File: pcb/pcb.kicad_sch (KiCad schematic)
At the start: 24 parts, among them U1 1117-3.3, U2 NORTH, U3 SOUTH, U4 EAST, U5 WEST

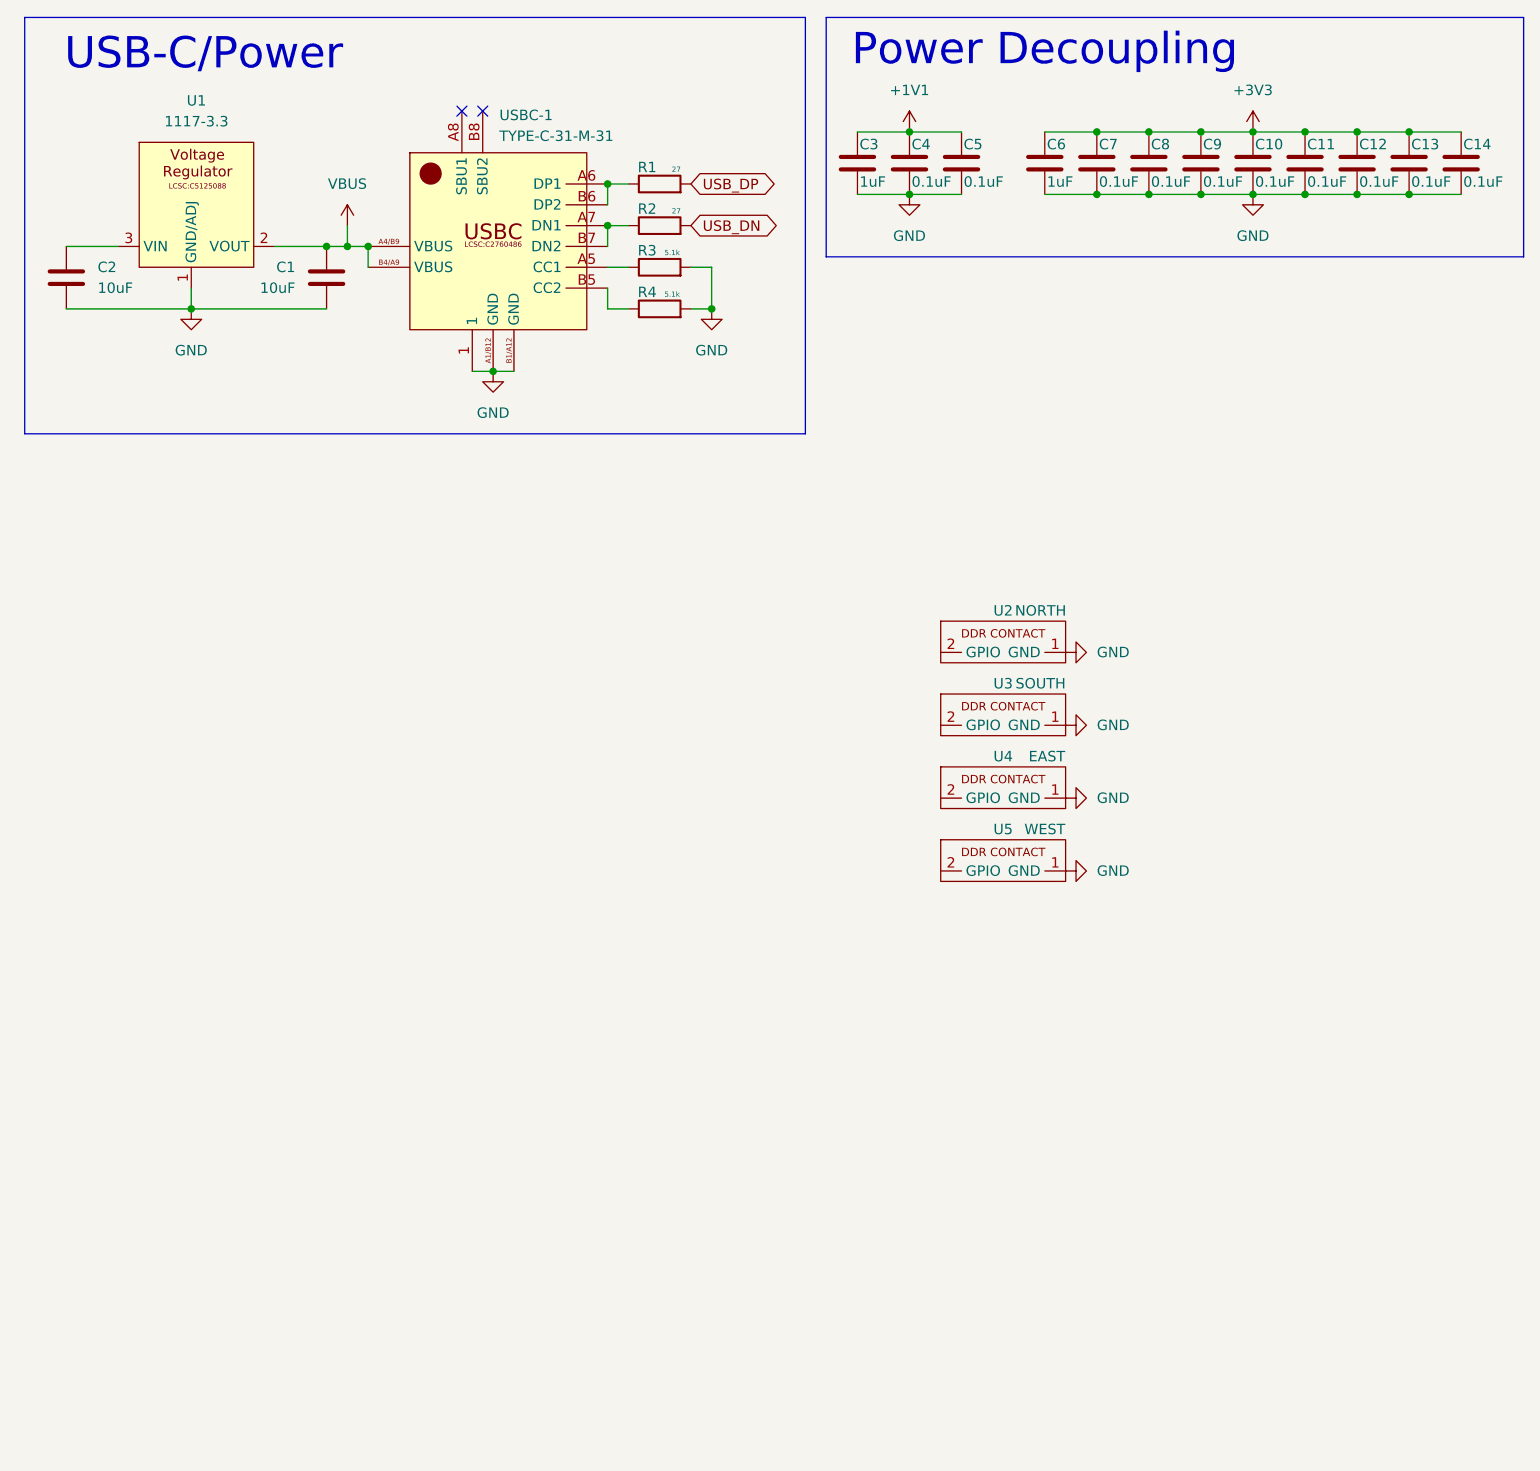
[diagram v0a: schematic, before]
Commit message: work on schematic more
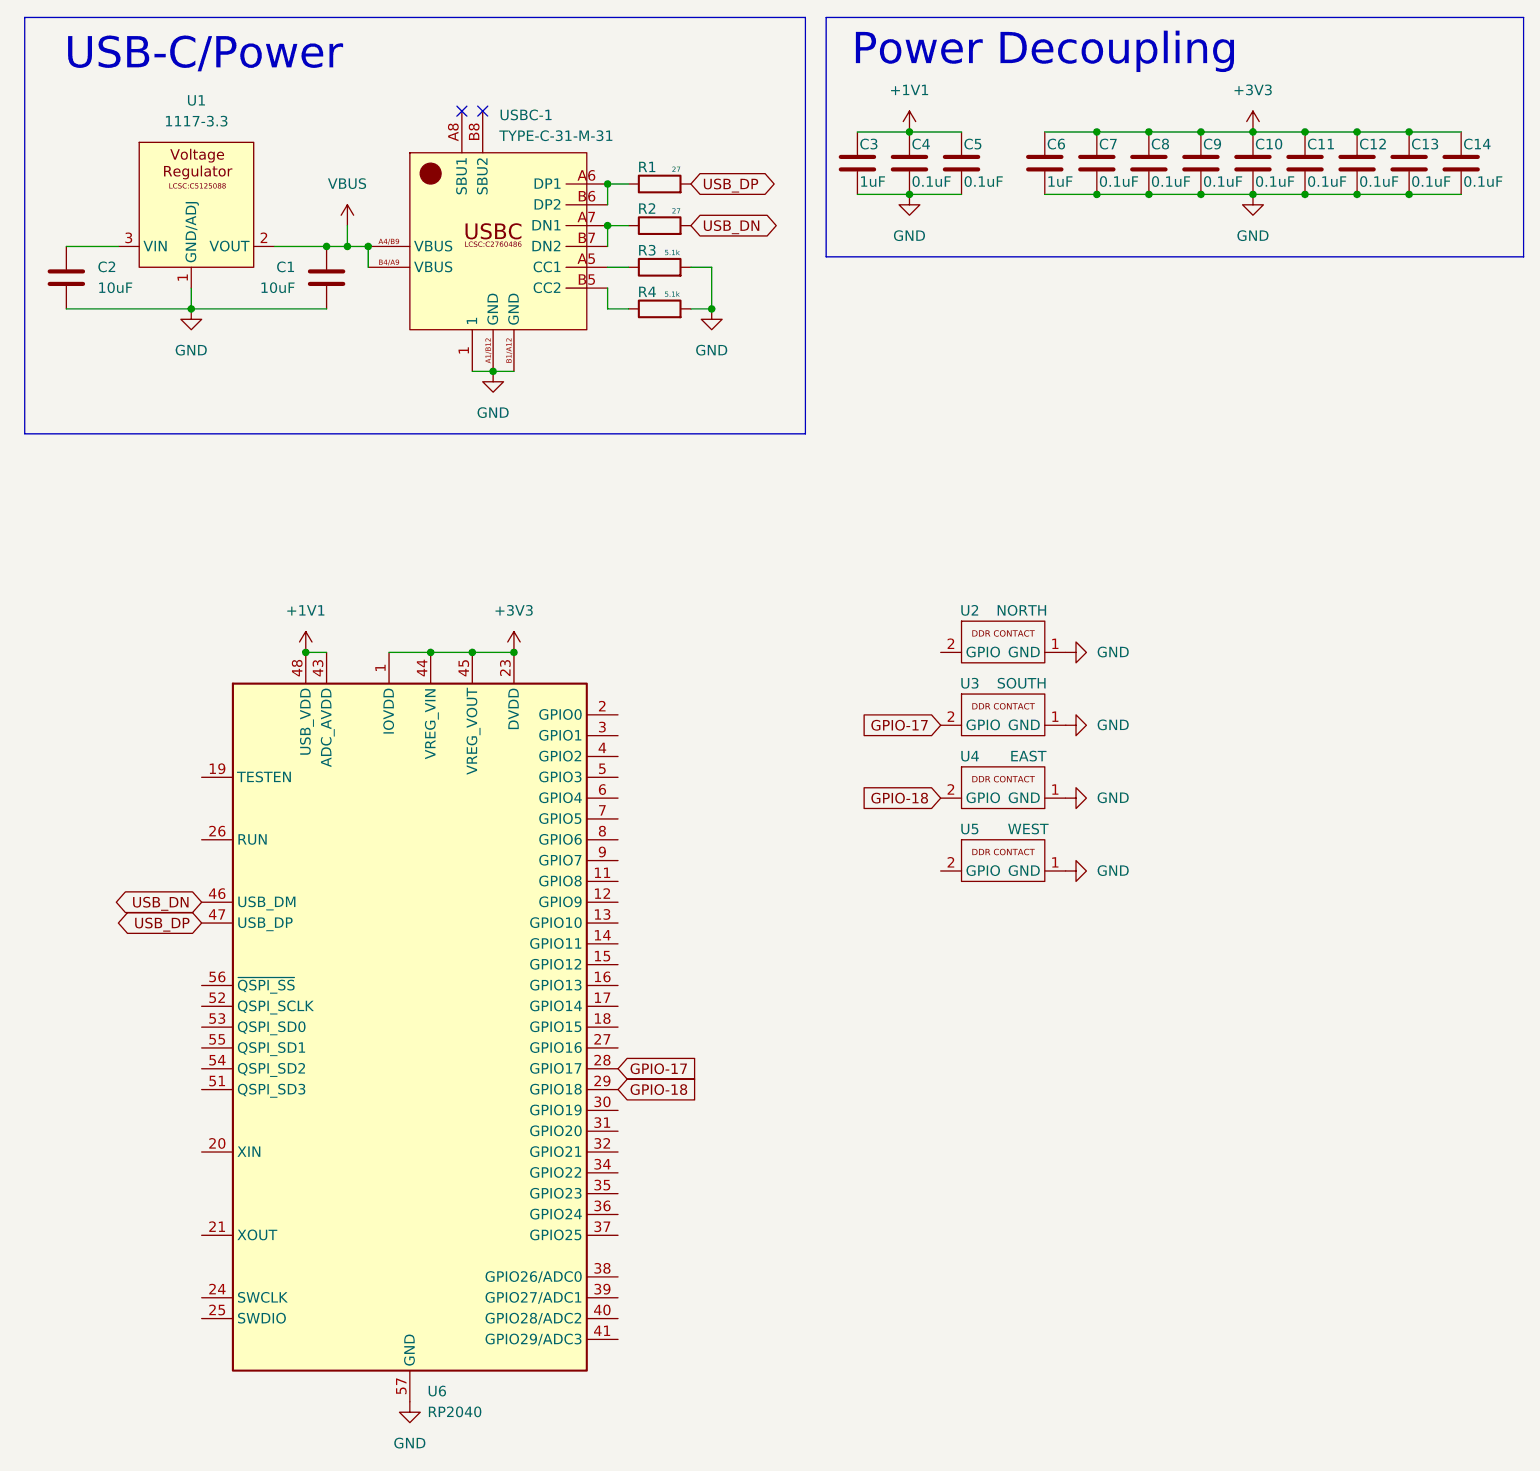
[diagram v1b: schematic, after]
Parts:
- added U6: RP2040, Package_DFN_QFN:QFN-56-1EP_7x7mm_P0.4mm_EP3.2x3.2mm, symbol MCU_RaspberryPi:RP2040
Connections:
- net +1V1: now also U6.43 (ADC_AVDD), U6.48 (USB_VDD)
- net +3V3: now also U6.1 (IOVDD), U6.10 (IOVDD), U6.22 (IOVDD), U6.23 (DVDD), U6.33 (IOVDD), U6.42 (IOVDD), U6.44 (VREG_VIN), U6.45 (VREG_VOUT), U6.49 (IOVDD), U6.50 (DVDD)
- net GND: now also U6.57 (GND)
- net USB_DN: now also U6.46 (USB_DM)
- net USB_DP: now also U6.47 (USB_DP)
- net GPIO-17: now reaches U3.2 (GPIO)
- net GPIO-17: now also U6.28 (GPIO17)
- net GPIO-18: now reaches U4.2 (GPIO)
- net GPIO-18: now also U6.29 (GPIO18)
